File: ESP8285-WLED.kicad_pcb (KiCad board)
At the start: 2 copper layers, 62.2 x 35.6 mm, 56 parts, among them J1 WLED, J2 USB_B_Micro, J3 ANT, Q1 UMH3N, SW1 RESET, SW2 FLASH, U1 ME3116, U2 ESP8285, U3 ME6211, U4 TXS0101, U5 CH340K, Y1 26MHz

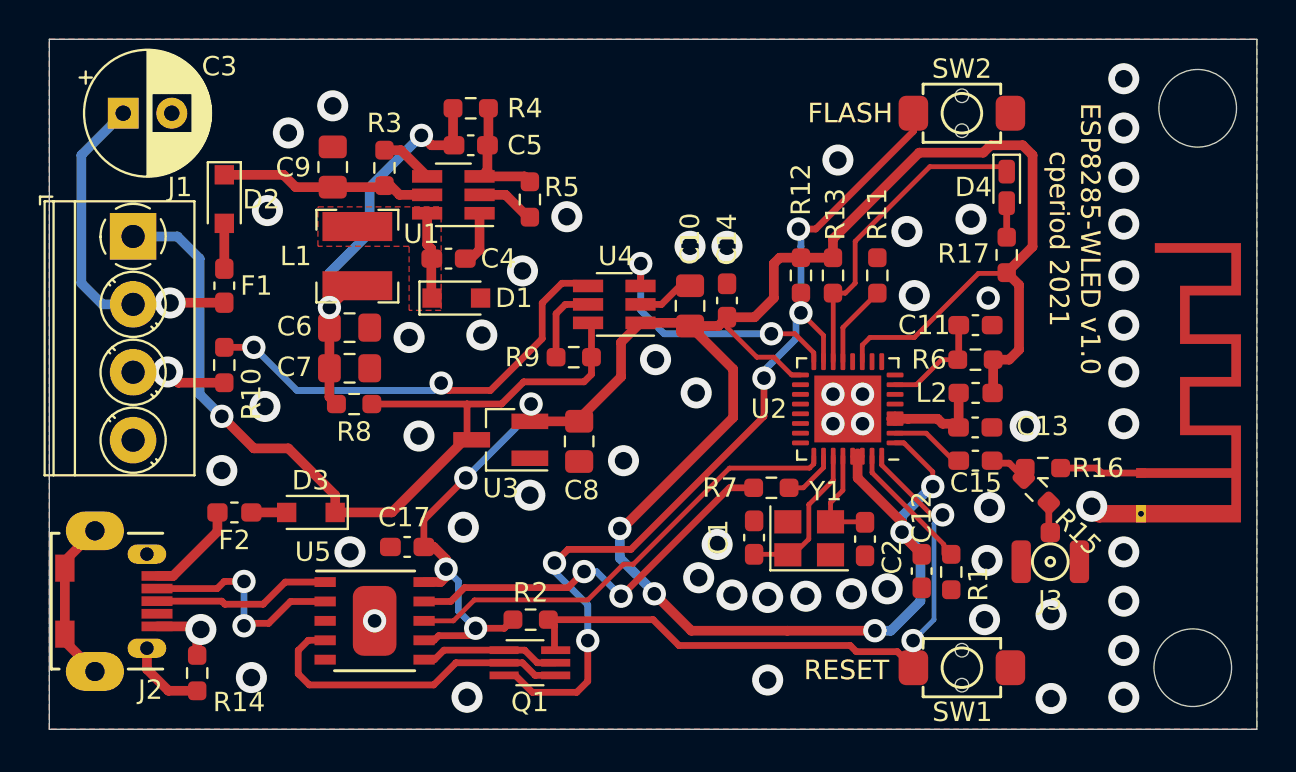
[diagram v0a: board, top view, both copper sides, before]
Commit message: even more tweaks
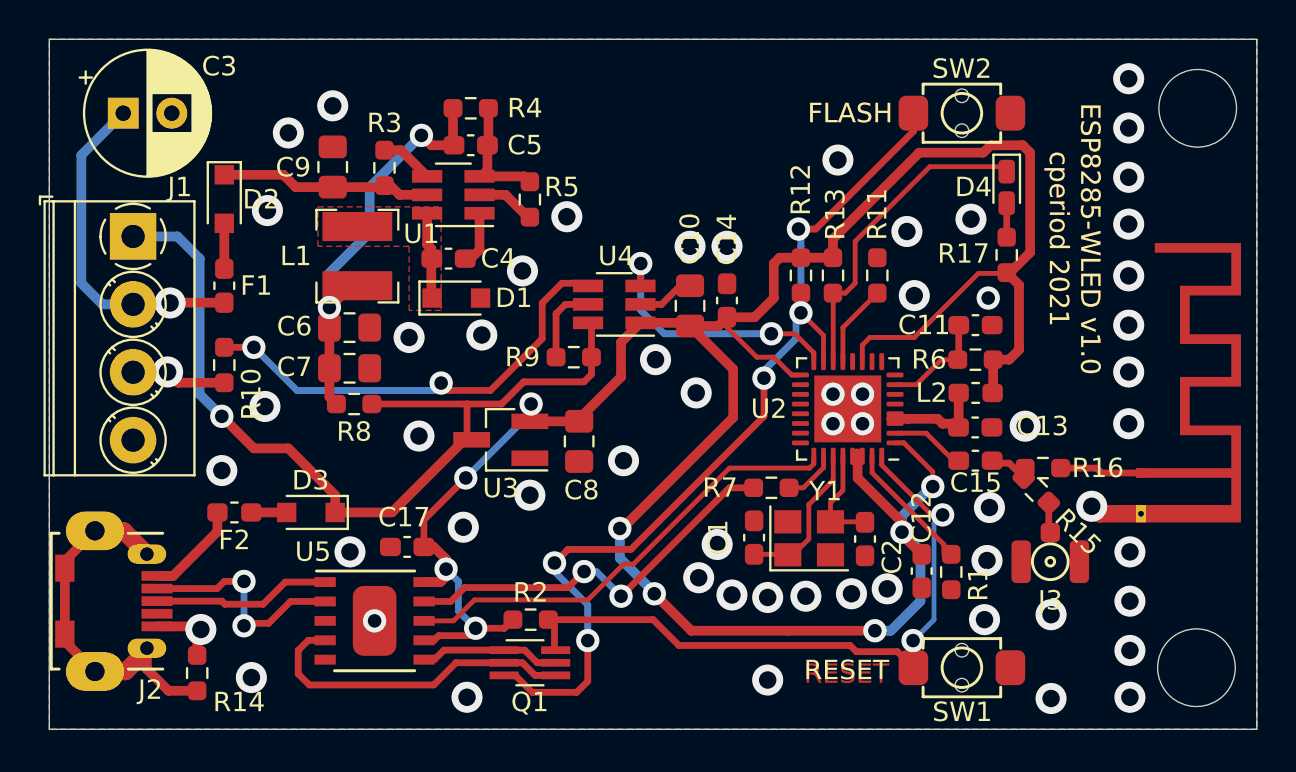
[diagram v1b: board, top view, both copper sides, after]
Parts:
- moved H1 0.19 mm to (149.3, 123.8)
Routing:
- net Net-(J2-Pad6): track 12.7 -> 19.1 mm
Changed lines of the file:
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@@
     (thickness 1.6)
     (drawings 14)
-    (tracks 441)
+    (tracks 447)
     (zones 0)
     (modules 56)
@@
   )
   (setup
-    (last_trace_width 0.25)
+    (last_trace_width 0.9)
     (user_trace_width 0.35)
     (user_trace_width 0.5)
@@
   )
   (module MountingHole:MountingHole_4mm (layer F.Cu)
-    (at 149.098 123.825)
+    (at 149.2885 123.825)
     (descr "Mounting Hole 4mm, no annular")
     (tags "mounting hole 4mm no annular")
@@
     (effects (font (size 2 2) (thickness 0.3)) (justify left mirror))
   )
-  (gr_text RESET (at 131.2545 123.952) (layer F.Cu)
+  (gr_text RESET (at 131.2545 124.1425) (layer F.Cu)
     (effects (font (size 1 1) (thickness 0.2)))
   )
@@
   (segment (start 113.68 99.456) (end 114.8315 100.6075) (width 0.5) (layer F.Cu) (net 2) (status 20))
   (segment (start 97.79 122.301) (end 97.79 122.301) (width 0.5) (layer F.Cu) (net 2) (status 20))
-  (via (at 145.542 111.252) (size 1.6) (drill 0.9) (layers F.Cu B.Cu) (net 2))
-  (via (at 145.542 108.585) (size 1.6) (drill 0.9) (layers F.Cu B.Cu) (net 2))
-  (via (at 145.542 106.172) (size 1.6) (drill 0.9) (layers F.Cu B.Cu) (net 2))
-  (via (at 145.542 103.632) (size 1.6) (drill 0.9) (layers F.Cu B.Cu) (net 2))
-  (via (at 145.542 100.965) (size 1.6) (drill 0.9) (layers F.Cu B.Cu) (net 2))
-  (via (at 145.542 98.552) (size 1.6) (drill 0.9) (layers F.Cu B.Cu) (net 2))
-  (via (at 145.542 120.396) (size 1.6) (drill 0.9) (layers F.Cu B.Cu) (net 2))
-  (via (at 145.542 122.936) (size 1.6) (drill 0.9) (layers F.Cu B.Cu) (net 2))
-  (via (at 145.542 125.349) (size 1.6) (drill 0.9) (layers F.Cu B.Cu) (net 2))
-  (via (at 145.542 96.012) (size 1.6) (drill 0.9) (layers F.Cu B.Cu) (net 2))
-  (via (at 145.542 93.472) (size 1.6) (drill 0.9) (layers F.Cu B.Cu) (net 2))
-  (via (at 145.542 117.856) (size 1.6) (drill 0.9) (layers F.Cu B.Cu) (net 2))
+  (via (at 145.796 111.252) (size 1.6) (drill 0.9) (layers F.Cu B.Cu) (net 2))
+  (via (at 145.796 108.585) (size 1.6) (drill 0.9) (layers F.Cu B.Cu) (net 2))
+  (via (at 145.796 100.965) (size 1.6) (drill 0.9) (layers F.Cu B.Cu) (net 2))
+  (via (at 145.796 98.552) (size 1.6) (drill 0.9) (layers F.Cu B.Cu) (net 2))
+  (via (at 145.8595 120.396) (size 1.6) (drill 0.9) (layers F.Cu B.Cu) (net 2))
+  (via (at 145.8595 122.936) (size 1.6) (drill 0.9) (layers F.Cu B.Cu) (net 2))
+  (via (at 145.8595 125.349) (size 1.6) (drill 0.9) (layers F.Cu B.Cu) (net 2))
+  (via (at 145.796 96.012) (size 1.6) (drill 0.9) (layers F.Cu B.Cu) (net 2))
+  (via (at 145.796 93.472) (size 1.6) (drill 0.9) (layers F.Cu B.Cu) (net 2))
+  (via (at 145.8595 117.856) (size 1.6) (drill 0.9) (layers F.Cu B.Cu) (net 2))
   (via (at 104.775 94.869) (size 1.6) (drill 0.9) (layers F.Cu B.Cu) (net 2))
   (via (at 102.489 96.266) (size 1.6) (drill 0.9) (layers F.Cu B.Cu) (net 2))
@@
   (via (at 123.5075 109.6645) (size 1.6) (drill 0.9) (layers F.Cu B.Cu) (net 2))
   (via (at 121.412 107.95) (size 1.6) (drill 0.9) (layers F.Cu B.Cu) (net 2))
+  (via (at 145.796 106.172) (size 1.6) (drill 0.9) (layers F.Cu B.Cu) (net 2))
+  (via (at 145.796 103.632) (size 1.6) (drill 0.9) (layers F.Cu B.Cu) (net 2))
   (segment (start 94.488 105.1) (end 92.908 105.1) (width 0.5) (layer B.Cu) (net 3) (status 10))
   (segment (start 92.908 105.1) (end 91.821 104.013) (width 0.5) (layer B.Cu) (net 3))
@@
   (segment (start 140.1445 107.442) (end 139.6365 107.95) (width 0.5) (layer F.Cu) (net 4))
   (segment (start 139.5095 103.465) (end 140.1445 104.1) (width 0.5) (layer F.Cu) (net 4))
-  (segment (start 140.843 102.1315) (end 139.5095 103.465) (width 0.5) (layer F.Cu) (net 4))
-  (segment (start 140.843 97.409) (end 140.843 102.1315) (width 0.5) (layer F.Cu) (net 4))
-  (segment (start 140.335 96.901) (end 140.843 97.409) (width 0.5) (layer F.Cu) (net 4))
-  (segment (start 138.303 97.282) (end 138.684 96.901) (width 0.5) (layer F.Cu) (net 4))
-  (segment (start 138.684 96.901) (end 140.335 96.901) (width 0.5) (layer F.Cu) (net 4))
-  (segment (start 130.556 101.727) (end 135.001 97.282) (width 0.5) (layer F.Cu) (net 4))
-  (segment (start 135.001 97.282) (end 138.303 97.282) (width 0.5) (layer F.Cu) (net 4))
-  (segment (start 130.556 102.696) (end 130.556 101.727) (width 0.5) (layer F.Cu) (net 4))
   (segment (start 138.049 103.505) (end 139.4695 103.505) (width 0.25) (layer F.Cu) (net 4))
   (segment (start 134.747 106.807) (end 138.049 103.505) (width 0.25) (layer F.Cu) (net 4))
@@
   (segment (start 119.6975 116.6495) (end 125.4125 110.9345) (width 0.5) (layer F.Cu) (net 4))
   (segment (start 119.5705 116.6495) (end 119.6975 116.6495) (width 0.5) (layer F.Cu) (net 4))
+  (segment (start 139.6765 103.465) (end 139.5095 103.465) (width 0.5) (layer F.Cu) (net 4))
+  (segment (start 140.716 102.4255) (end 139.6765 103.465) (width 0.5) (layer F.Cu) (net 4))
+  (segment (start 140.716 97.282) (end 140.716 102.4255) (width 0.5) (layer F.Cu) (net 4))
+  (segment (start 140.335 96.901) (end 140.716 97.282) (width 0.5) (layer F.Cu) (net 4))
+  (segment (start 138.684 96.901) (end 140.335 96.901) (width 0.5) (layer F.Cu) (net 4))
+  (segment (start 138.303 97.282) (end 138.684 96.901) (width 0.5) (layer F.Cu) (net 4))
+  (segment (start 135.001 97.282) (end 138.303 97.282) (width 0.5) (layer F.Cu) (net 4))
+  (segment (start 130.556 101.727) (end 135.001 97.282) (width 0.5) (layer F.Cu) (net 4))
+  (segment (start 130.556 102.696) (end 130.556 101.727) (width 0.5) (layer F.Cu) (net 4))
   (segment (start 137.036 107.9) (end 136.986 107.95) (width 0.35) (layer F.Cu) (net 5) (status 30))
   (segment (start 137.036 106.172) (end 137.036 107.9) (width 0.35) (layer F.Cu) (net 5) (status 30))
@@
   (segment (start 90.97 122.471) (end 92.52 124.021) (width 0.5) (layer F.Cu) (net 14) (status 30))
   (segment (start 90.97 122.096) (end 90.97 122.471) (width 0.5) (layer F.Cu) (net 14) (status 30))
+  (segment (start 94 116.771) (end 95.2 117.971) (width 0.9) (layer F.Cu) (net 14))
+  (segment (start 92.52 116.771) (end 94 116.771) (width 0.9) (layer F.Cu) (net 14))
+  (segment (start 95.2 122.821) (end 95.2 122.9225) (width 0.9) (layer F.Cu) (net 14))
+  (segment (start 94.1015 124.021) (end 92.52 124.021) (width 0.9) (layer F.Cu) (net 14))
+  (segment (start 95.2 122.9225) (end 94.1015 124.021) (width 0.9) (layer F.Cu) (net 14))
   (segment (start 141.678735 116.786735) (end 141.756 116.864) (width 0.35) (layer F.Cu) (net 15))
   (segment (start 141.678735 115.326235) (end 141.678735 116.786735) (width 0.35) (layer F.Cu) (net 15))
